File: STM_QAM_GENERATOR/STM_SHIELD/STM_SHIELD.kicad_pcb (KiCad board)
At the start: 2 copper layers, 2 parts, among them U1 NUCLEO-F446RE, U2 ADA4807-2ARM

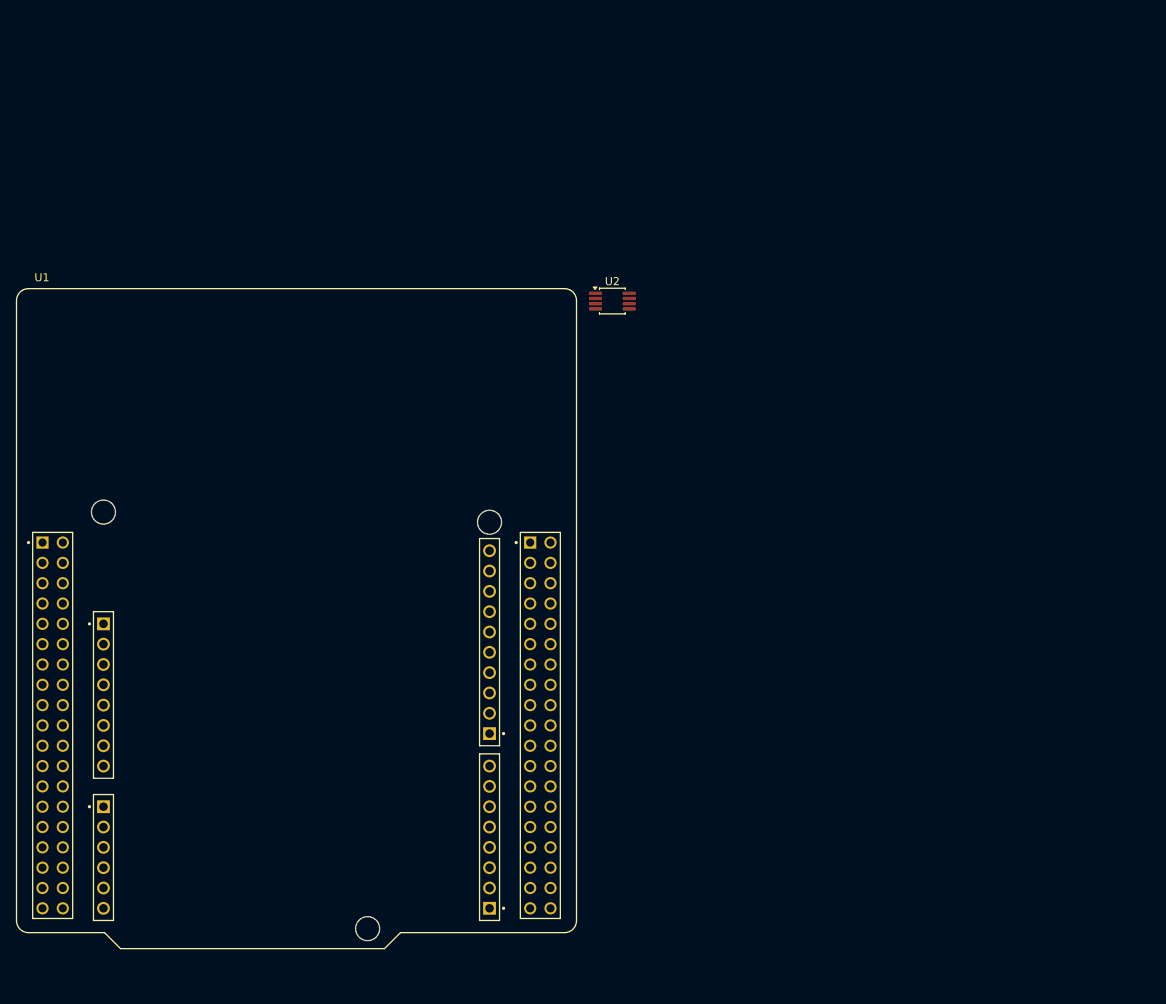
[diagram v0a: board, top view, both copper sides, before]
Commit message: STM_SHIELD_DONE
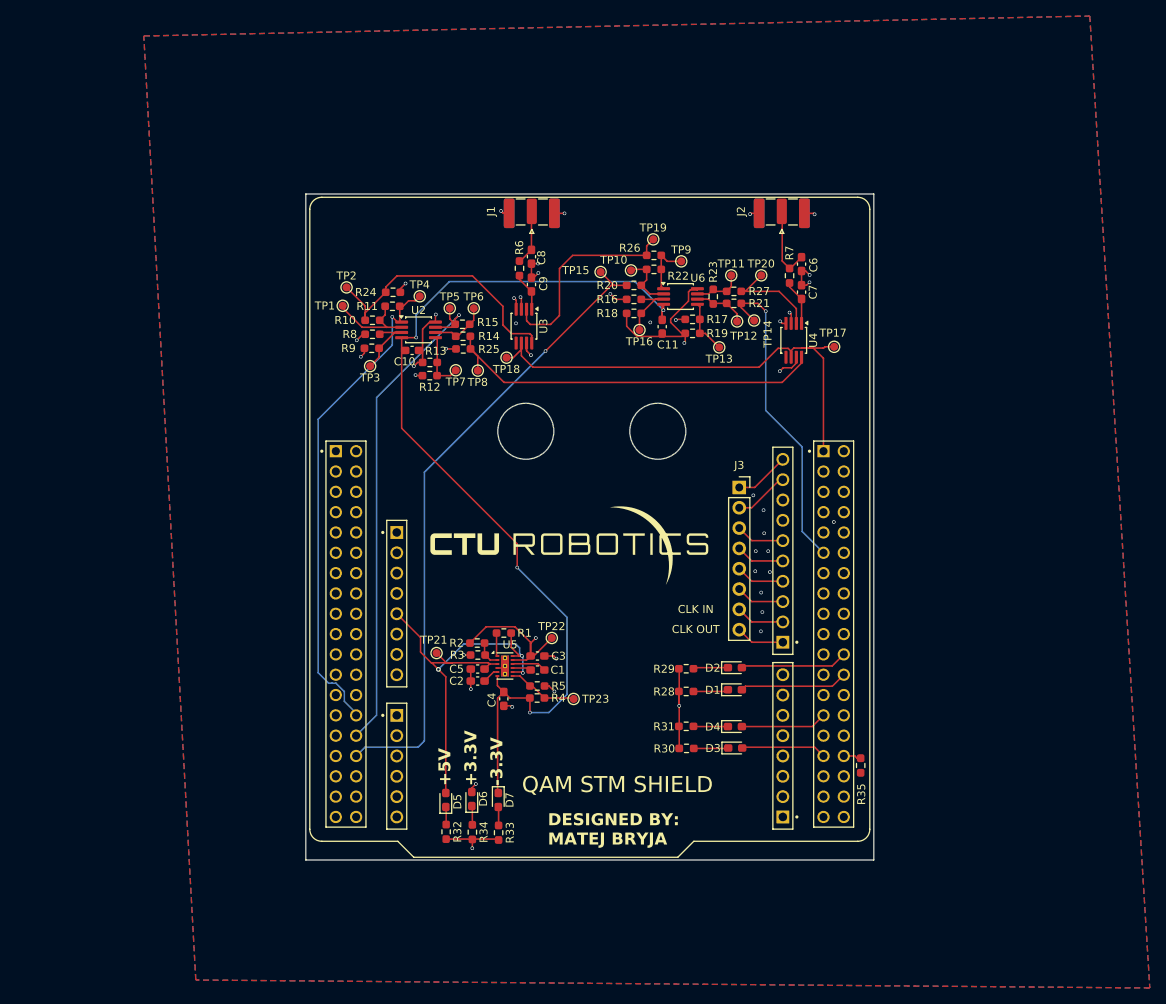
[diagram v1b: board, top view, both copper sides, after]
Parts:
- added C1: C, Capacitor_SMD:C_0603_1608Metric_Pad1.08x0.95mm_HandSolder, F.Cu at (130.2, 120.8)
- added C10: C, Capacitor_SMD:C_0603_1608Metric_Pad1.08x0.95mm_HandSolder, F.Cu at (114.5, 80.8)
- added C11: C, Capacitor_SMD:C_0603_1608Metric_Pad1.08x0.95mm_HandSolder, F.Cu at (145.8, 77.8)
- added C2: C, Capacitor_SMD:C_0603_1608Metric_Pad1.08x0.95mm_HandSolder, F.Cu at (122.7, 122.1)
- added C3: C, Capacitor_SMD:C_0603_1608Metric_Pad1.08x0.95mm_HandSolder, F.Cu at (130.2, 119.0)
- added C4: C, Capacitor_SMD:C_0603_1608Metric_Pad1.08x0.95mm_HandSolder, F.Cu at (126.0, 124.4)
- added C5: C, Capacitor_SMD:C_0603_1608Metric_Pad1.08x0.95mm_HandSolder, F.Cu at (122.7, 120.6)
- added C6: C, Capacitor_SMD:C_0603_1608Metric_Pad1.08x0.95mm_HandSolder, F.Cu at (163.2, 70.0)
- added C7: C, Capacitor_SMD:C_0603_1608Metric_Pad1.08x0.95mm_HandSolder, F.Cu at (163.2, 73.5)
- added C8: C, Capacitor_SMD:C_0603_1608Metric_Pad1.08x0.95mm_HandSolder, F.Cu at (129.5, 69.1)
- added C9: C, Capacitor_SMD:C_0603_1608Metric_Pad1.08x0.95mm_HandSolder, F.Cu at (129.5, 72.6)
- added D1: LED, LED_SMD:LED_0603_1608Metric_Pad1.05x0.95mm_HandSolder, F.Cu at (154.9, 123.2)
- added D2: LED, LED_SMD:LED_0603_1608Metric_Pad1.05x0.95mm_HandSolder, F.Cu at (154.9, 120.5)
- added D3: LED, LED_SMD:LED_0603_1608Metric_Pad1.05x0.95mm_HandSolder, F.Cu at (154.9, 130.5)
- added D4: LED, LED_SMD:LED_0603_1608Metric_Pad1.05x0.95mm_HandSolder, F.Cu at (154.9, 127.8)
- added D5: LED, LED_SMD:LED_0603_1608Metric_Pad1.05x0.95mm_HandSolder, F.Cu at (118.8, 137.0)
- added D6: LED, LED_SMD:LED_0603_1608Metric_Pad1.05x0.95mm_HandSolder, F.Cu at (122.0, 136.9)
- added D7: LED, LED_SMD:LED_0603_1608Metric_Pad1.05x0.95mm_HandSolder, F.Cu at (125.3, 137.0)
- added J1: SMA_I, Connector_Coaxial:SMA_Samtec_SMA-J-P-H-ST-EM1_EdgeMount, F.Cu at (129.5, 63.4)
- added J2: SMA_Q, Connector_Coaxial:SMA_Samtec_SMA-J-P-H-ST-EM1_EdgeMount, F.Cu at (160.8, 63.4)
- added J3: Conn_01x08_Socket, Connector_PinSocket_2.54mm:PinSocket_1x08_P2.54mm_Vertical, F.Cu at (155.4, 97.9)
- added R1: R, Resistor_SMD:R_0603_1608Metric_Pad0.98x0.95mm_HandSolder, F.Cu at (126.0, 116.1)
- added R10: R, Resistor_SMD:R_0603_1608Metric_Pad0.98x0.95mm_HandSolder, F.Cu at (109.6, 77.0)
- added R11: R, Resistor_SMD:R_0603_1608Metric_Pad0.98x0.95mm_HandSolder, F.Cu at (112.1, 75.3)
- added R12: R, Resistor_SMD:R_0603_1608Metric_Pad0.98x0.95mm_HandSolder, F.Cu at (116.7, 84.0)
- added R13: R, Resistor_SMD:R_0603_1608Metric_Pad0.98x0.95mm_HandSolder, F.Cu at (116.8, 82.3)
- added R14: R, Resistor_SMD:R_0603_1608Metric_Pad0.98x0.95mm_HandSolder, F.Cu at (120.9, 79.0)
- added R15: R, Resistor_SMD:R_0603_1608Metric_Pad0.98x0.95mm_HandSolder, F.Cu at (120.8, 77.5)
- added R16: R, Resistor_SMD:R_0603_1608Metric_Pad0.98x0.95mm_HandSolder, F.Cu at (142.3, 74.4)
- added R17: R, Resistor_SMD:R_0603_1608Metric_Pad0.98x0.95mm_HandSolder, F.Cu at (149.6, 76.9)
- added R18: R, Resistor_SMD:R_0603_1608Metric_Pad0.98x0.95mm_HandSolder, F.Cu at (142.3, 76.2)
- added R19: R, Resistor_SMD:R_0603_1608Metric_Pad0.98x0.95mm_HandSolder, F.Cu at (149.6, 78.7)
- added R2: R, Resistor_SMD:R_0603_1608Metric_Pad0.98x0.95mm_HandSolder, F.Cu at (122.7, 117.4)
- added R20: R, Resistor_SMD:R_0603_1608Metric_Pad0.98x0.95mm_HandSolder, F.Cu at (142.3, 72.7)
- added R21: R, Resistor_SMD:R_0603_1608Metric_Pad0.98x0.95mm_HandSolder, F.Cu at (154.8, 74.9)
- added R22: R, Resistor_SMD:R_0603_1608Metric_Pad0.98x0.95mm_HandSolder, F.Cu at (144.8, 70.7)
- added R23: R, Resistor_SMD:R_0603_1608Metric_Pad0.98x0.95mm_HandSolder, F.Cu at (152.2, 74.1)
- added R24: R, Resistor_SMD:R_0603_1608Metric_Pad0.98x0.95mm_HandSolder, F.Cu at (112.2, 73.5)
- added R25: R, Resistor_SMD:R_0603_1608Metric_Pad0.98x0.95mm_HandSolder, F.Cu at (120.9, 80.6)
- added R26: R, Resistor_SMD:R_0603_1608Metric_Pad0.98x0.95mm_HandSolder, F.Cu at (144.8, 68.9)
- added R27: R, Resistor_SMD:R_0603_1608Metric_Pad0.98x0.95mm_HandSolder, F.Cu at (154.8, 73.4)
- added R28: R, Resistor_SMD:R_0603_1608Metric_Pad0.98x0.95mm_HandSolder, F.Cu at (148.8, 123.4)
- added R29: R, Resistor_SMD:R_0603_1608Metric_Pad0.98x0.95mm_HandSolder, F.Cu at (148.8, 120.6)
- added R3: R, Resistor_SMD:R_0603_1608Metric_Pad0.98x0.95mm_HandSolder, F.Cu at (122.8, 118.9)
- added R30: R, Resistor_SMD:R_0603_1608Metric_Pad0.98x0.95mm_HandSolder, F.Cu at (148.8, 130.6)
- added R31: R, Resistor_SMD:R_0603_1608Metric_Pad0.98x0.95mm_HandSolder, F.Cu at (148.8, 127.8)
- added R32: R, Resistor_SMD:R_0603_1608Metric_Pad0.98x0.95mm_HandSolder, F.Cu at (118.8, 141.0)
- added R33: R, Resistor_SMD:R_0603_1608Metric_Pad0.98x0.95mm_HandSolder, F.Cu at (125.3, 141.1)
- added R34: R, Resistor_SMD:R_0603_1608Metric_Pad0.98x0.95mm_HandSolder, F.Cu at (122.1, 141.0)
- added R35: DNP, Resistor_SMD:R_0603_1608Metric_Pad0.98x0.95mm_HandSolder, F.Cu at (170.6, 132.7)
- added R4: R, Resistor_SMD:R_0603_1608Metric_Pad0.98x0.95mm_HandSolder, F.Cu at (130.2, 124.2)
- added R5: R, Resistor_SMD:R_0603_1608Metric_Pad0.98x0.95mm_HandSolder, F.Cu at (130.2, 122.8)
- added R6: R, Resistor_SMD:R_0603_1608Metric_Pad0.98x0.95mm_HandSolder, F.Cu at (128.0, 70.5)
- added R7: R, Resistor_SMD:R_0603_1608Metric_Pad0.98x0.95mm_HandSolder, F.Cu at (161.7, 71.5)
- added R8: R, Resistor_SMD:R_0603_1608Metric_Pad0.98x0.95mm_HandSolder, F.Cu at (109.6, 78.8)
- added R9: R, Resistor_SMD:R_0603_1608Metric_Pad0.98x0.95mm_HandSolder, F.Cu at (109.5, 80.5)
- added REF**: CTU_LOGO, Custom:CTU_LOGO, F.Cu at (132.5, 104.8)
- added TP1: TestPoint, TestPoint:TestPoint_Pad_D1.0mm, F.Cu at (105.9, 75.2)
- added TP10: TestPoint, TestPoint:TestPoint_Pad_D1.0mm, F.Cu at (141.9, 70.8)
- added TP11: TestPoint, TestPoint:TestPoint_Pad_D1.0mm, F.Cu at (154.4, 71.4)
- added TP12: TestPoint, TestPoint:TestPoint_Pad_D1.0mm, F.Cu at (155.2, 77.2)
- added TP13: TestPoint, TestPoint:TestPoint_Pad_D1.0mm, F.Cu at (152.9, 80.4)
- added TP14: TestPoint, TestPoint:TestPoint_Pad_D1.0mm, F.Cu at (157.3, 77.1)
- added TP15: TestPoint, TestPoint:TestPoint_Pad_D1.0mm, F.Cu at (138.1, 71.0)
- added TP16: TestPoint, TestPoint:TestPoint_Pad_D1.0mm, F.Cu at (143.0, 78.2)
- added TP17: TestPoint, TestPoint:TestPoint_Pad_D1.0mm, F.Cu at (167.3, 80.3)
- added TP18: TestPoint, TestPoint:TestPoint_Pad_D1.0mm, F.Cu at (126.3, 81.7)
- added TP19: TestPoint, TestPoint:TestPoint_Pad_D1.0mm, F.Cu at (144.7, 66.9)
- added TP2: TestPoint, TestPoint:TestPoint_Pad_D1.0mm, F.Cu at (106.3, 72.9)
- added TP20: TestPoint, TestPoint:TestPoint_Pad_D1.0mm, F.Cu at (158.2, 71.4)
- added TP21: TestPoint, TestPoint:TestPoint_Pad_D1.0mm, F.Cu at (117.6, 118.6)
- added TP22: TestPoint, TestPoint:TestPoint_Pad_D1.0mm, F.Cu at (132.0, 116.8)
- added TP23: TestPoint, TestPoint:TestPoint_Pad_D1.0mm, F.Cu at (134.7, 124.4)
- added TP3: TestPoint, TestPoint:TestPoint_Pad_D1.0mm, F.Cu at (109.3, 82.8)
- added TP4: TestPoint, TestPoint:TestPoint_Pad_D1.0mm, F.Cu at (115.5, 74.0)
- added TP5: TestPoint, TestPoint:TestPoint_Pad_D1.0mm, F.Cu at (119.2, 75.5)
- added TP6: TestPoint, TestPoint:TestPoint_Pad_D1.0mm, F.Cu at (122.2, 75.5)
- added TP7: TestPoint, TestPoint:TestPoint_Pad_D1.0mm, F.Cu at (120.0, 83.3)
- added TP8: TestPoint, TestPoint:TestPoint_Pad_D1.0mm, F.Cu at (122.8, 83.3)
- added TP9: TestPoint, TestPoint:TestPoint_Pad_D1.0mm, F.Cu at (148.2, 69.7)
- added U3: ADG619, Package_SO:MSOP-8_3x3mm_P0.65mm, F.Cu at (128.5, 77.8)
- added U4: ADG619, Package_SO:MSOP-8_3x3mm_P0.65mm, F.Cu at (162.2, 79.5)
- added U5: LM27762, Package_SON:WSON-12-1EP_3x2mm_P0.5mm_EP1x2.65_ThermalVias, F.Cu at (126.1, 120.2)
- added U6: ADA4807-2ARM, Package_SO:MSOP-8_3x3mm_P0.65mm, F.Cu at (148.1, 74.1)
- moved U1 38.4 mm to (136.8, 102.9)
- moved U2 24.5 mm to (115.3, 78.2)
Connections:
- U1 pad CN10_1: unconnected-(U1B-PC9-PadCN10_1) -> RX/TX
- U1 pad CN10_11: unconnected-(U1B-PA5-PadCN10_11) -> DAC_Q
- U1 pad CN10_20: CN10_GND -> GND
- U1 pad CN10_22: unconnected-(U1B-PB2-PadCN10_22) -> Net-(D2-A)
- U1 pad CN10_24: unconnected-(U1B-PB1-PadCN10_24) -> Net-(D1-A)
- U1 pad CN10_27: unconnected-(U1B-PB4-PadCN10_27) -> Net-(D4-A)
- U1 pad CN10_31: unconnected-(U1B-PB3-PadCN10_31) -> Net-(D3-A)
- U1 pad CN10_32: unconnected-(U1B-AGND-PadCN10_32) -> Net-(U1B-AGND)
- U1 pad CN10_9: CN10_GND -> GND
- U1 pad CN5_1: unconnected-(U1F-D8-PadCN5_1) -> Net-(J3-Pin_8)
- U1 pad CN5_10: unconnected-(U1F-D15-PadCN5_10) -> Net-(J3-Pin_1)
- U1 pad CN5_2: unconnected-(U1F-D9-PadCN5_2) -> Net-(J3-Pin_7)
- U1 pad CN5_3: unconnected-(U1F-D10-PadCN5_3) -> Net-(J3-Pin_6)
- U1 pad CN5_4: unconnected-(U1F-D11-PadCN5_4) -> Net-(J3-Pin_5)
- U1 pad CN5_5: unconnected-(U1F-D12-PadCN5_5) -> Net-(J3-Pin_4)
- U1 pad CN5_6: unconnected-(U1F-D13-PadCN5_6) -> Net-(J3-Pin_3)
- U1 pad CN5_7: unconnected-(U1F-CN5_GND-PadCN5_7) -> GND
- U1 pad CN5_9: unconnected-(U1F-D14-PadCN5_9) -> Net-(J3-Pin_2)
- U1 pad CN6_5: unconnected-(U1C-CN6_+5V-PadCN6_5) -> +5V
- U1 pad CN6_6: CN6_GND -> GND
- U1 pad CN6_7: CN6_GND -> GND
- U1 pad CN7_19: CN7_GND -> GND
- U1 pad CN7_20: CN7_GND -> GND
- U1 pad CN7_22: CN7_GND -> GND
- U1 pad CN7_28: unconnected-(U1A-PA0-PadCN7_28) -> ADC_I
- U1 pad CN7_30: unconnected-(U1A-PA1-PadCN7_30) -> ADC_Q
- U1 pad CN7_32: unconnected-(U1A-PA4-PadCN7_32) -> DAC_I
- U1 pad CN7_8: CN7_GND -> GND
- U2 pad 1: unconnected-(U2-Pad1) -> ADC_I
- U2 pad 2: unconnected-(U2A---Pad2) -> Net-(U2A--)
- U2 pad 3: unconnected-(U2A-+-Pad3) -> Net-(U2A-+)
- U2 pad 4: unconnected-(U2C-V--Pad4) -> -3.3V
- U2 pad 5: unconnected-(U2B-+-Pad5) -> Net-(U2B-+)
- U2 pad 6: unconnected-(U2B---Pad6) -> Net-(U2B--)
- U2 pad 7: unconnected-(U2-Pad7) -> ADC_Q
- U2 pad 8: unconnected-(U2C-V+-Pad8) -> +3.3V
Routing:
- net -3.3V: track 0.00 -> 122.2 mm, vias 0 -> 4
- net DAC_I: track 0.00 -> 80.2 mm, vias 0 -> 1
- net ADC_Q: track 0.00 -> 64.6 mm, vias 0 -> 1
- net ADC_I: track 0.00 -> 62.7 mm, vias 0 -> 1
- net RX/TX: track 0.00 -> 62.1 mm
- net GND: track 0.00 -> 57.4 mm, vias 0 -> 38
- net +5V: track 0.00 -> 57.3 mm, vias 0 -> 3
- net +3.3V: track 0.00 -> 52.2 mm, vias 0 -> 8
- net RX_Q: track 0.00 -> 49.5 mm
- net DAC_Q: track 0.00 -> 39.5 mm, vias 0 -> 1
- net RX_I: track 0.00 -> 34.5 mm
- net TX_I: track 0.00 -> 26.0 mm
- net Net-(D1-A): track 0.00 -> 13.5 mm
- net Net-(D2-A): track 0.00 -> 13.4 mm
- net TX_Q: track 0.00 -> 13.0 mm
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- added copper zone on In2.Cu, net +3.3V
- added copper zone on B.Cu, net GND
- added copper zone on F.Cu, net GND
- added copper zone on In1.Cu, net GND
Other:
- board outline added: 71 x 83.2 mm
- copper layers 2 -> 4
- board text added: "+3.3V"
- board text added: "+5V"
- board text added: "-3.3V"
- board text added: "CLK IN"
- board text added: "CLK OUT"
- board text added: "DESIGNED BY: MATEJ BRYJA"
- board text added: "QAM STM SHIELD"
